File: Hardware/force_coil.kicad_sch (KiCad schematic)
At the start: 22 parts

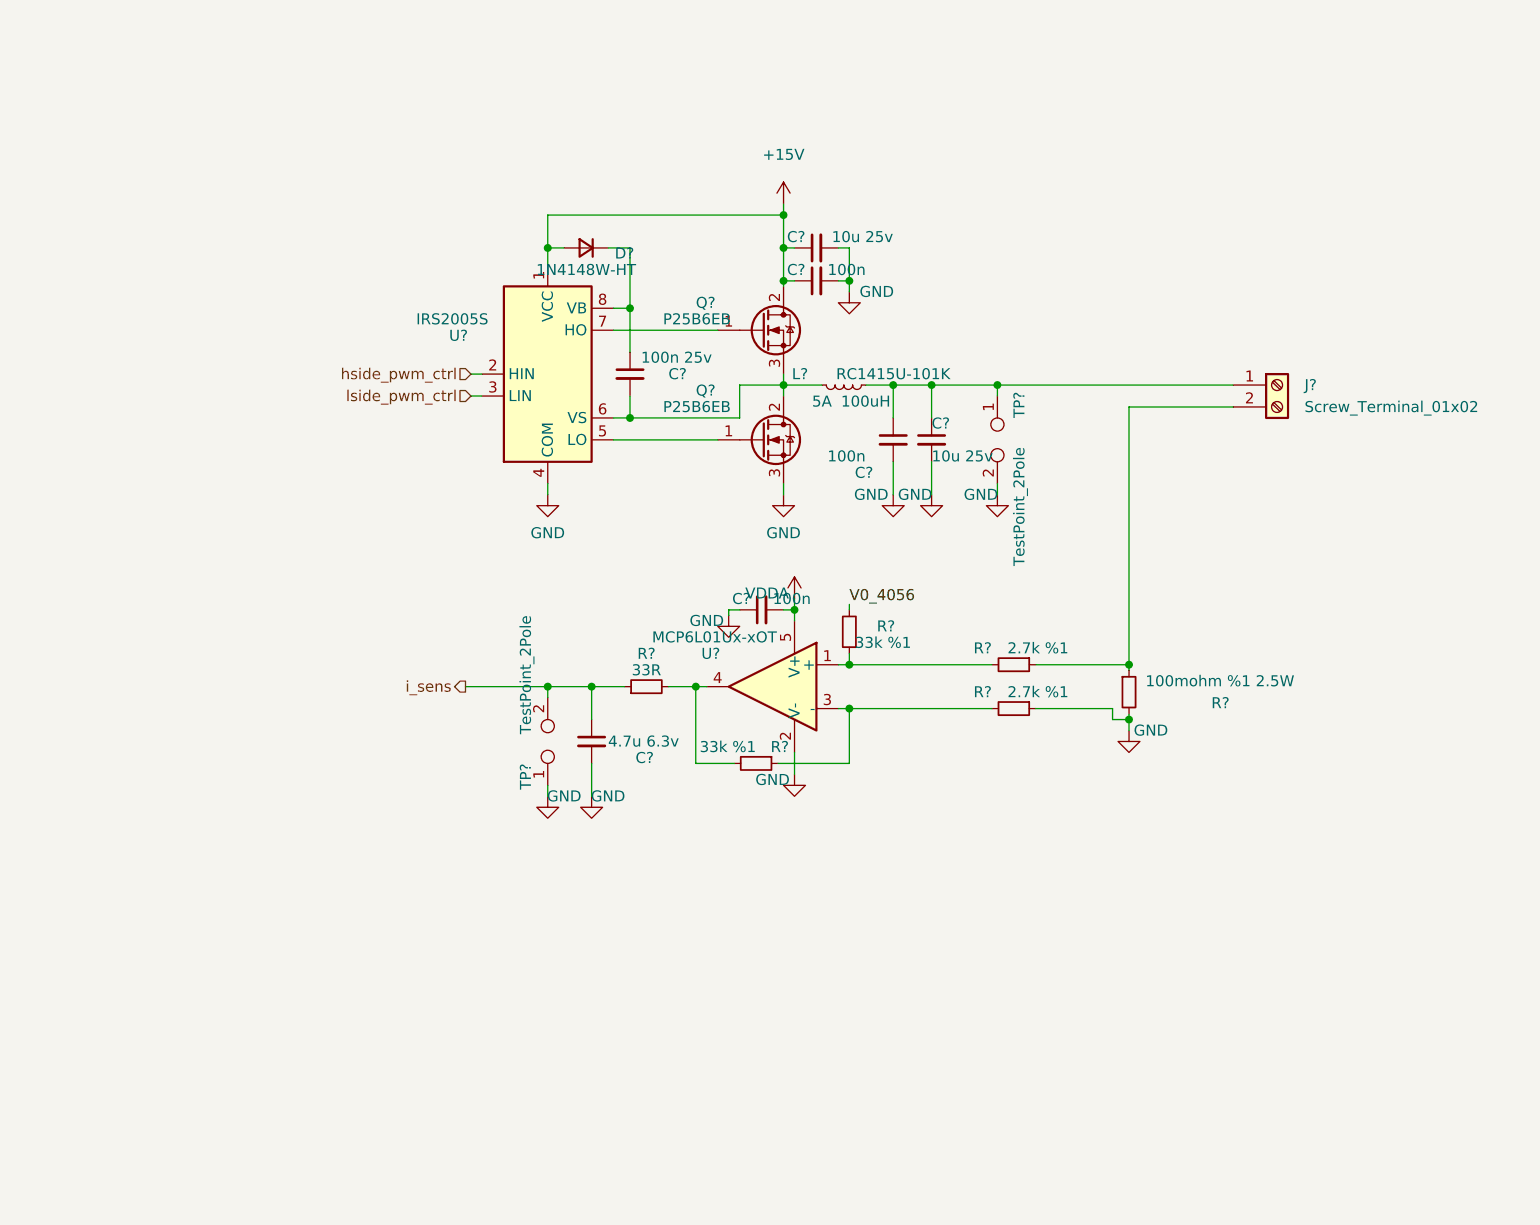
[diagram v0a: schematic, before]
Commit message: Completed schematic and PCB.
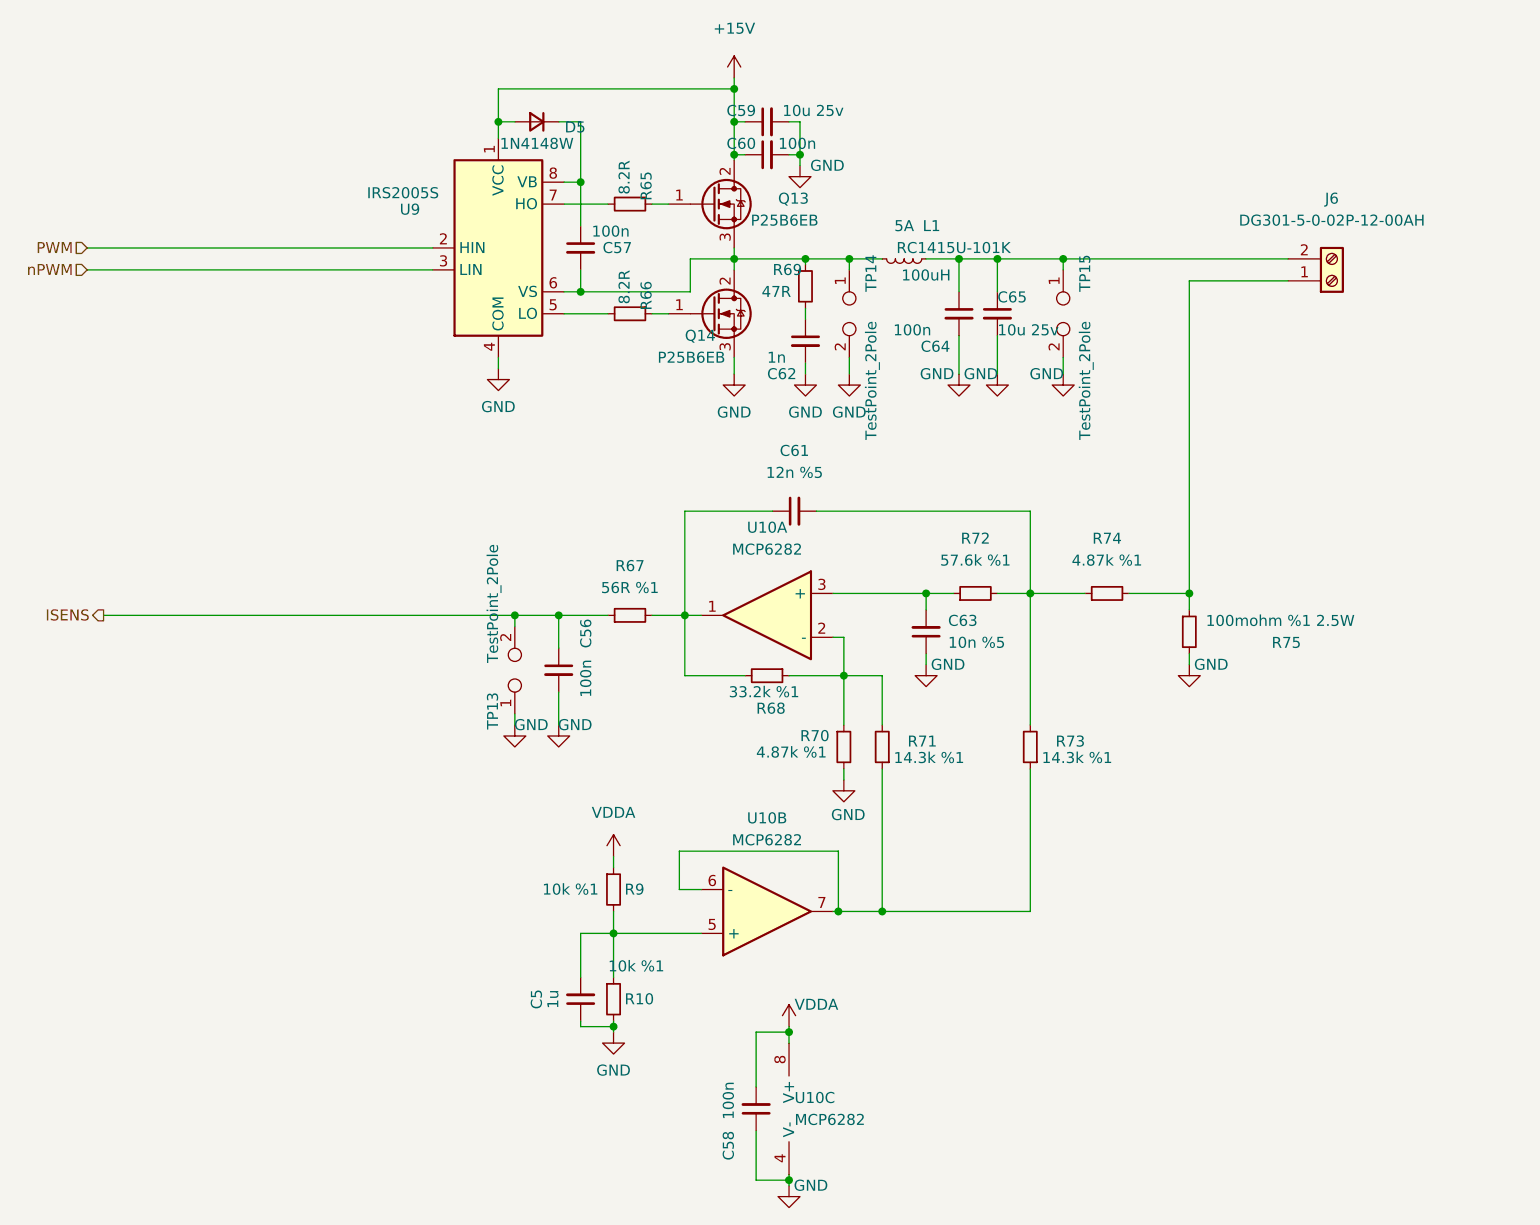
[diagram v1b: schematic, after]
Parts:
- removed C?: 4.7u 6.3v, Capacitor_SMD:C_0603_1608Metric_Pad1.08x0.95mm_HandSolder, symbol Device:C_Small
- removed C?: 100n, Capacitor_SMD:C_0603_1608Metric_Pad1.08x0.95mm_HandSolder, symbol Device:C_Small
- removed J?: Screw_Terminal_01x02, symbol Connector:Screw_Terminal_01x02
- removed R? (x2): 2.7k %1, Resistor_SMD:R_0603_1608Metric_Pad0.98x0.95mm_HandSolder, symbol Device:R_Small
- removed R?: 33R, Resistor_SMD:R_0603_1608Metric_Pad0.98x0.95mm_HandSolder, symbol Device:R_Small
- removed R? (x2): 33k %1, Resistor_SMD:R_0603_1608Metric_Pad0.98x0.95mm_HandSolder, symbol Device:R_Small
- removed TP?: TestPoint_2Pole, Connector_PinHeader_2.54mm:PinHeader_1x02_P2.54mm_Vertical, symbol Connector:TestPoint_2Pole
- removed U?: MCP6L01Ux-xOT, Package_TO_SOT_SMD:SOT-23-5, symbol Amplifier_Operational:MCP6L01Ux-xOT
- added C5: 1u, Capacitor_SMD:C_0603_1608Metric_Pad1.08x0.95mm_HandSolder, symbol Device:C_Small
- added C56, C58: 100n, Capacitor_SMD:C_0603_1608Metric_Pad1.08x0.95mm_HandSolder, symbol Device:C_Small
- added C61: 12n %5, Capacitor_SMD:C_0805_2012Metric_Pad1.18x1.45mm_HandSolder, symbol Device:C_Small
- added C62: 1n, Capacitor_SMD:C_0603_1608Metric_Pad1.08x0.95mm_HandSolder, symbol Device:C_Small
- added C63: 10n %5, Capacitor_SMD:C_0603_1608Metric_Pad1.08x0.95mm_HandSolder, symbol Device:C_Small
- added J6: DG301-5-0-02P-12-00AH, conn:DG301-5.0-02P-12-00AH, symbol Connector:Screw_Terminal_01x02
- added R10, R9: 10k %1, Resistor_SMD:R_0603_1608Metric_Pad0.98x0.95mm_HandSolder, symbol Device:R_Small
- added R65, R66: 8.2R, Resistor_SMD:R_0603_1608Metric_Pad0.98x0.95mm_HandSolder, symbol Device:R_Small
- added R67: 56R %1, Resistor_SMD:R_0603_1608Metric_Pad0.98x0.95mm_HandSolder, symbol Device:R_Small
- added R68: 33.2k %1, Resistor_SMD:R_0603_1608Metric_Pad0.98x0.95mm_HandSolder, symbol Device:R_Small
- added R69: 47R, Resistor_SMD:R_0603_1608Metric_Pad0.98x0.95mm_HandSolder, symbol Device:R_Small
- added R70, R74: 4.87k %1, Resistor_SMD:R_0603_1608Metric_Pad0.98x0.95mm_HandSolder, symbol Device:R_Small
- added R71, R73: 14.3k %1, Resistor_SMD:R_0603_1608Metric_Pad0.98x0.95mm_HandSolder, symbol Device:R_Small
- added R72: 57.6k %1, Resistor_SMD:R_0603_1608Metric_Pad0.98x0.95mm_HandSolder, symbol Device:R_Small
- added TP13, TP14: TestPoint_2Pole, Connector_PinHeader_2.54mm:PinHeader_1x02_P2.54mm_Vertical, symbol Connector:TestPoint_2Pole
- added U10: MCP6282, Package_SO:SOIC-8_3.9x4.9mm_P1.27mm, symbol Device:Opamp_Dual
- C57: renamed from C?; value 100n 25v -> 100n
- D5: renamed from D?; value 1N4148W-HT -> 1N4148W
- L1: renamed from L?; footprint (none) -> inductor:RC1415U-101K
- Q13, Q14: renamed from Q?; footprint Package_TO_SOT_SMD:TO-252-3_TabPin2 -> Package_TO_SOT_SMD:TO-252-2
- TP15: renamed from TP?; Link https://ozdisan.com/connectors-and-interconnects/headers/pin-headers/C2100-02ASGAS0R -> https://ozdisan.com/connectors-and-interconnects/headers/pin-headers/L-KLS1-207-1-02-S
- gave numbers to parts that had none: 6
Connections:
- net GND: now also C5.1, C56.2, C58.1, C62.2, C63.1, R10.2, R70.2, TP13.1, TP14.2, U10.4 (V-)
- net VDDA: now also C58.2, R9.1, U10.8 (V+)
- net at R75.1: now also J6.1 (Pin_1), R74.2
- net at C64.1, C65.1, L1.1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: now also J6.2 (Pin_2)
- net at C57.2, L1.2, Q13.3 (S)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: now also R69.1, TP14.1
- net at Q14.1 (G): now also R66.1; no longer U9.5 (LO)
- net at Q13.1 (G): now also R65.1; no longer U9.7 (HO)
- net hside_pwm_ctrl renamed PWM
- net lside_pwm_ctrl renamed nPWM
- new net: C63.2, R72.1, U10.3 (+)
- new net: C61.2, R72.2, R73.2, R74.1
- new net: C62.1, R69.2
- new net: C61.1, R67.2, R68.2, U10.1
- new net: R68.1, R70.1, R71.2, U10.2 (-)
- new net: C5.2, R10.1, R9.2, U10.5 (+)
- new net: R71.1, R73.1, U10.6 (-), U10.7
- new net: R66.2, U9.5 (LO)
- new net: R65.2, U9.7 (HO)
- new net ISENS: C56.1, R67.1, TP13.2
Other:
- moved on the sheet: C57, C59, C60, C64, C65, D5, L1, Q13, Q14, R75, TP15, U9
